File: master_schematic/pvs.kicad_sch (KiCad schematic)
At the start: 70 parts, among them J11 1723103102, J12 1723103102, J13 1723103102, J14 1723103102, J15 1723103102, J16 1723103102, J17 1723103102, J18 1723103102, J19 1723103102, J20 1723103102, J54 1723103102, J55 1723103102, J56 1723103102, J57 1723103102, J58 1723103102, J59 1723103102, J60 1723103102, J61 1723103102, J62 1723103102, J63 1723103102, J64 1722563102, J65 1722563102, J66 1722563102, J67 1722563102, J68 1722563102, J69 1722563102, J70 1722563102, J71 1722563102, J72 1722563102, J73 1722563102, J74 1722563102, J75 1722563102, J76 1722563102, J77 1722563102, J78 1722563102, J79 1722563102, J80 1722563102, J81 1722563102, J82 1722563102, J83 1722563102, Q1 CWDM3011N TR13 PBFREE, Q10 CWDM3011N TR13 PBFREE, Q2 CWDM3011N TR13 PBFREE, Q3 CWDM3011N TR13 PBFREE, Q4 CWDM3011N TR13 PBFREE, Q5 CWDM3011N TR13 PBFREE, Q6 CWDM3011N TR13 PBFREE, Q7 CWDM3011N TR13 PBFREE, Q8 CWDM3011N TR13 PBFREE, Q9 CWDM3011N TR13 PBFREE

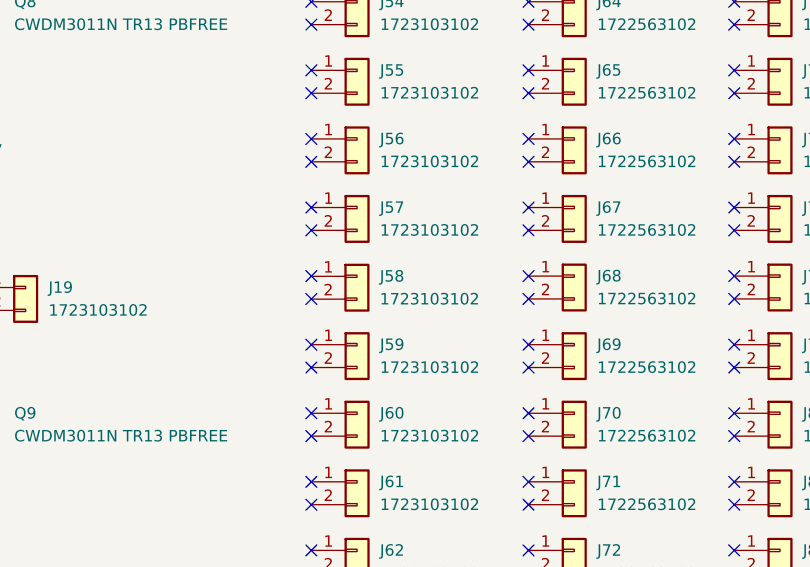
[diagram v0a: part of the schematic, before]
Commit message: stuff
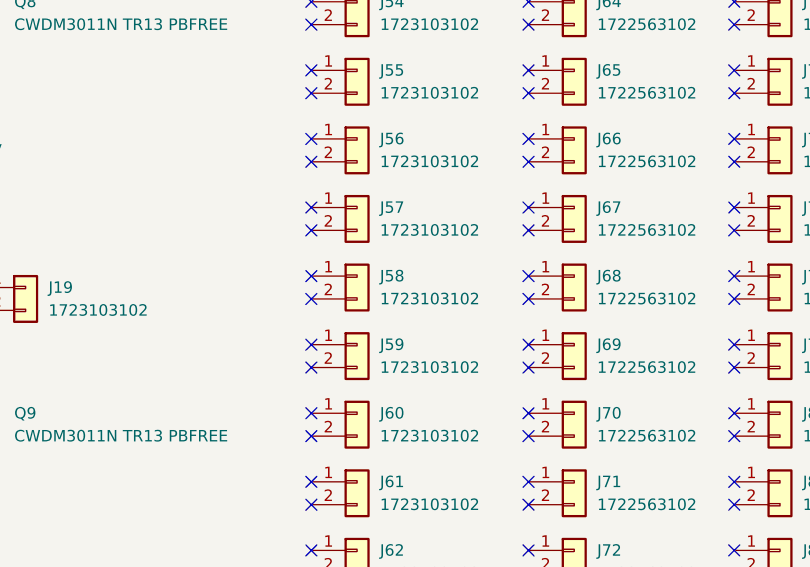
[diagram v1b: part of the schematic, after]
